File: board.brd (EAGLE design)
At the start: 53.3 x 33.5 mm, 86 parts, among them J1 AVR_SPI_PRG_6NS, U1 TPS2112A, U2 MAX1555, U3 USD-SOCKETNEW, U4 3.3V, U5 2.8V, U6 74HC595, Y1 8MHz, Y2 12.288MHz

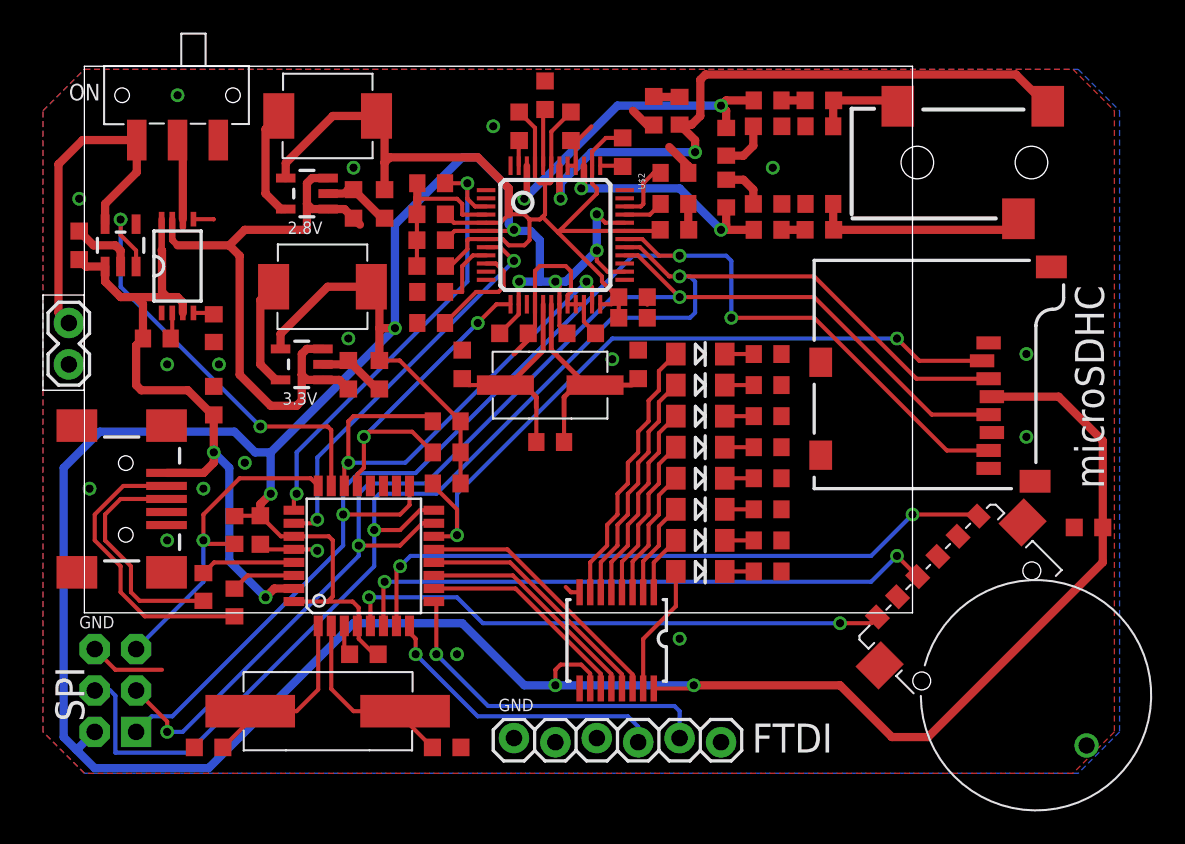
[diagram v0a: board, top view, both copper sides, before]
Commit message: More board cleanup
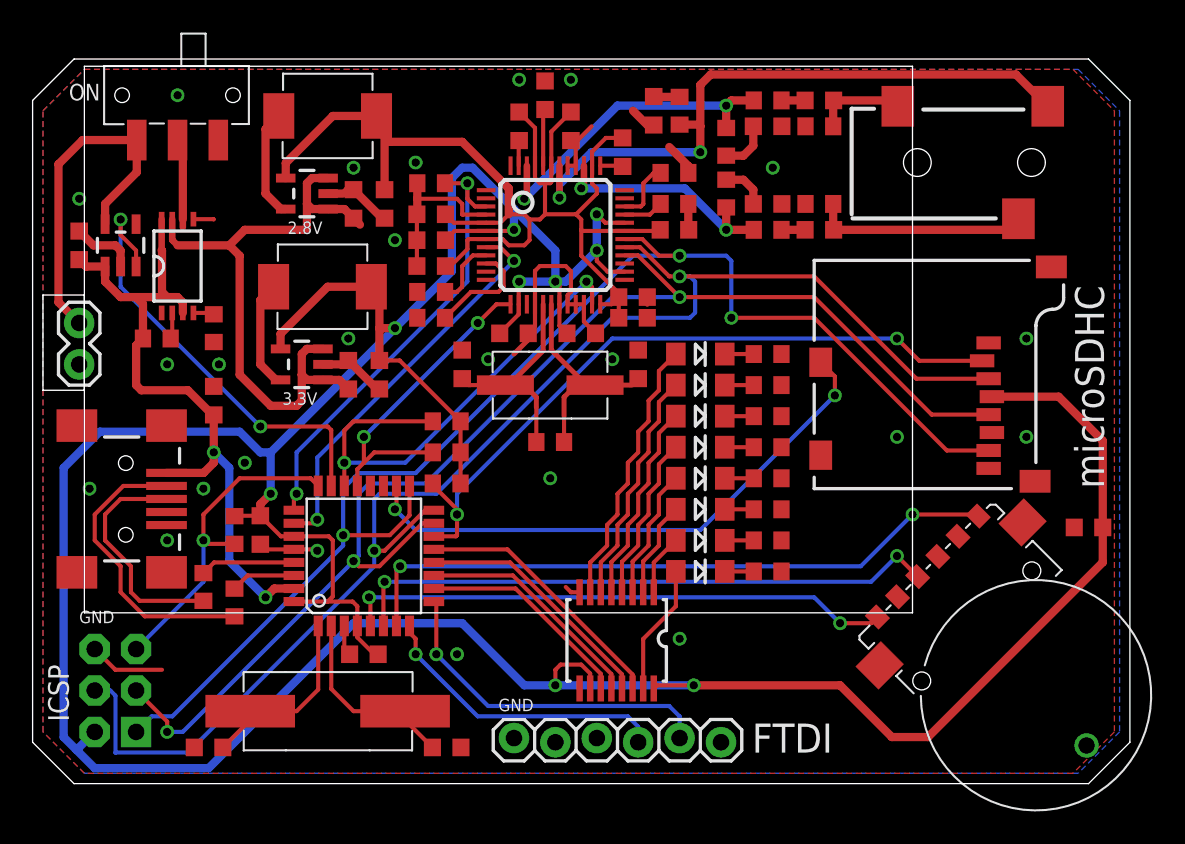
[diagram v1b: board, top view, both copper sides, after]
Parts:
- C25: value 1u -> 0.1u
- moved JP3 0.64 mm to (2.22, 27.6)
- moved R13 0.32 mm to (23.8, 27.9)
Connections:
- net SD_CD: now also U$1.18
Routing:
- net SD_CD: track 0.00 -> 34.8 mm, vias 0 -> 2
- net SD_CS: track 44.5 -> 43.2 mm
- net CVDD: track 73.4 -> 72.1 mm
- net SCK: track 79.9 -> 80.9 mm
- net MISO: track 82.7 -> 83.6 mm
- net VDD: track 233.9 -> 233.3 mm
- net GND: vias 18 -> 24
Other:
- board size 53.3 x 33.5 mm -> 67.3 x 44.4 mm
- board text added: "ICSP"
- board text added: "MJK 09/13"
- board text added: "mattkeeter.com"
- board text removed: "MJK 09/13 mattkeeter.com"
- board text removed: "SPI"
